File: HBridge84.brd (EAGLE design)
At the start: 53.3 x 40.6 mm, 21 parts, among them J5 ICSP

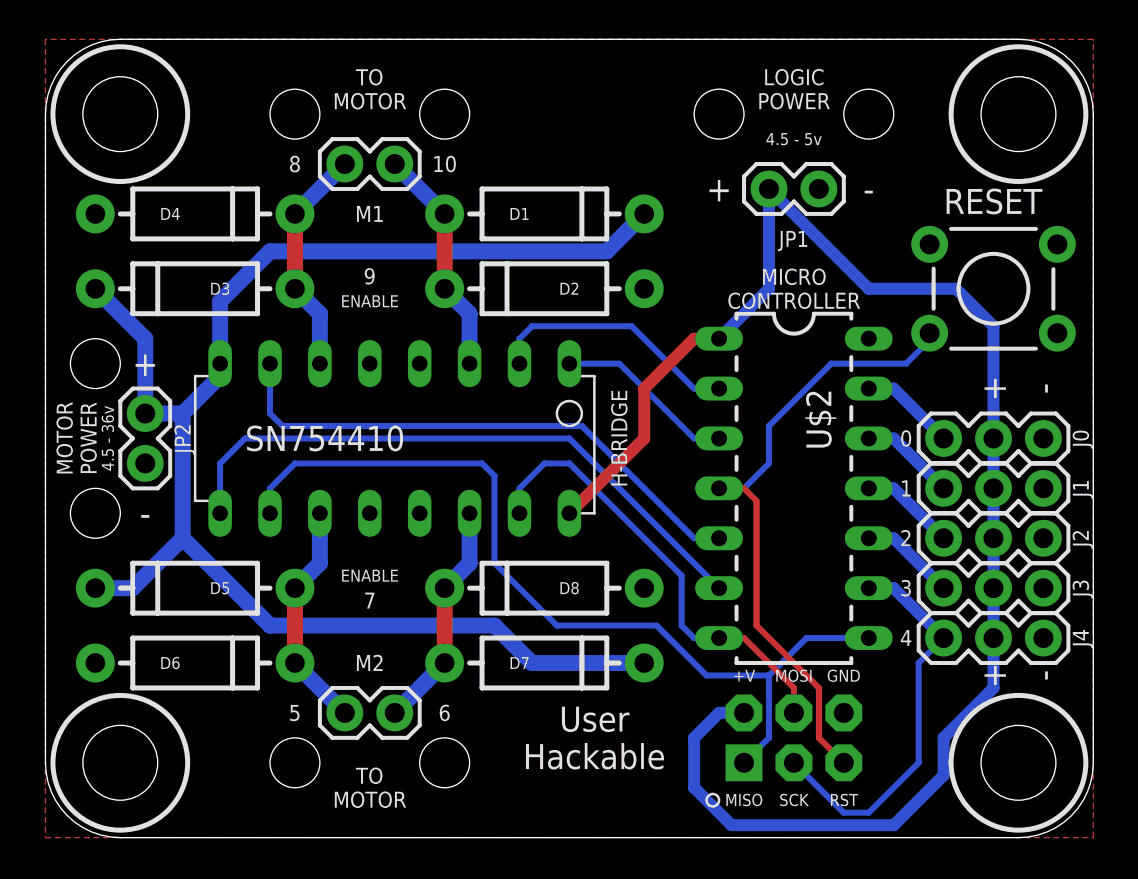
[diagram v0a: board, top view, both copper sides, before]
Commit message: adding eagle files
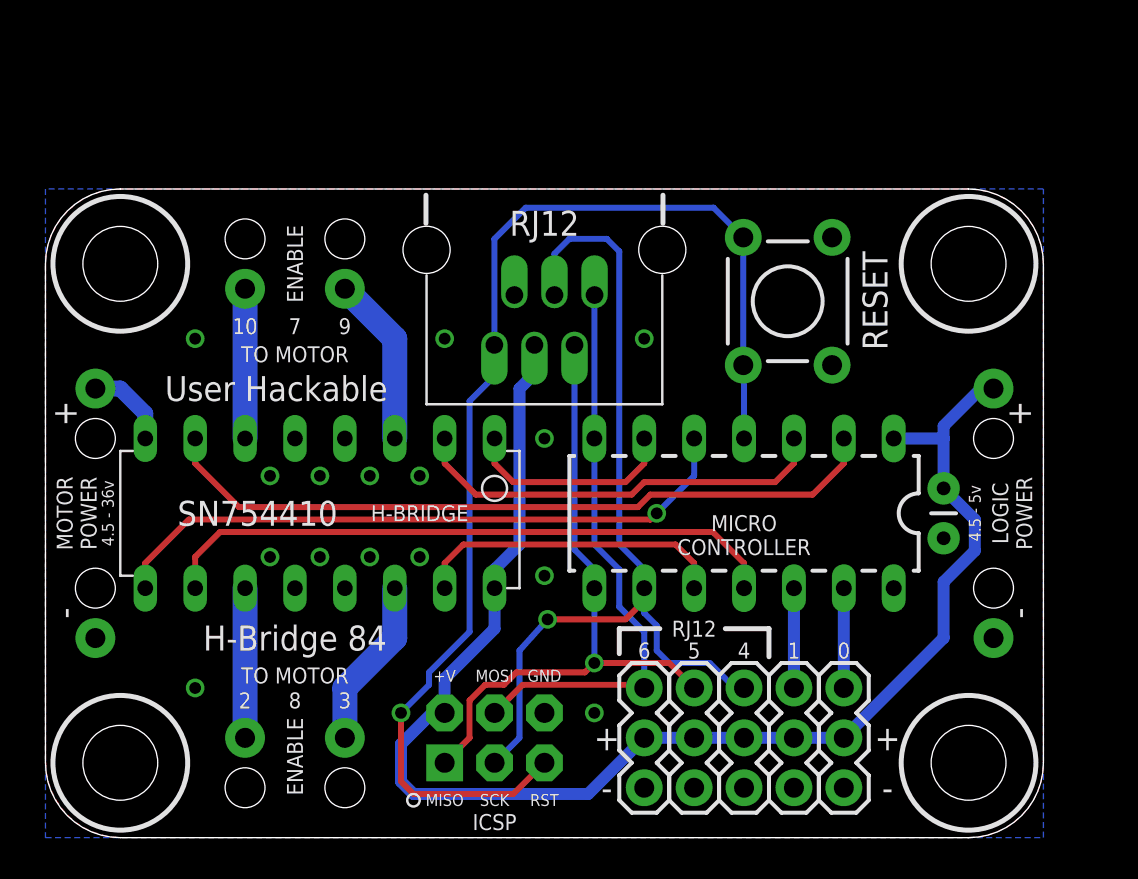
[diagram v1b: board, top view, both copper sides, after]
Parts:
- removed D1, D2, D3, D4, D5, D6, D7, D8: (no value), SparkFun-DiscreteSemi:DIODE-1N4001
- removed JP1, JP2, M1, M2: (no value), SparkFun-Connectors:1X02
- added C2: (no value), barbary_enterprises:CAP-PTH-SMALL
- added U$1, U$10, U$3, U$4, U$5, U$6, U$8, U$9: M1, barbary_enterprises:M1_NO_STRAIN
- added U$7: RJ12, barbary_enterprises:RJ12
- moved J4 21.7 mm to (30.5, 2.54), turned to 90 degrees
- moved J0 20.5 mm to (40.6, 2.54), turned to 90 degrees
- moved J3 20.5 mm to (33.0, 2.54), turned to 90 degrees
- moved J1 19.8 mm to (38.1, 2.54), turned to 90 degrees
- moved J2 19.8 mm to (35.6, 2.54), turned to 90 degrees
- moved J5 15.2 mm to (22.9, 5.08)
- moved RESET 10.5 mm to (37.8, 27.3), turned to 270 degrees
- moved SN754410 5.39 mm to (14.0, 16.5)
- moved U$2 3.81 mm to (34.3, 16.5), turned to 180 degrees
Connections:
- net 10: now also SN754410.7; no longer SN754410.2
- net 2: now also SN754410.10; no longer J2.3
- net 3: now also SN754410.15; no longer J3.3
- net 4: now also J2.3, U$7.4; no longer J4.3
- net 5: now also J3.3, U$7.5; no longer SN754410.10
- net 5V: now also C2.1, U$10.P$1, U$7.3; no longer JP1.2
- net 6: now also J4.3, U$7.6; no longer SN754410.15
- net 7: now also SN754410.1; no longer SN754410.9
- net 8: now also SN754410.9; no longer SN754410.7
- net 9: now also SN754410.2; no longer SN754410.1
- net GND: now also C2.2, RESET.1, U$7.2, U$8.P$1, U$9.P$1; no longer D2.A, D4.A, D6.A, D8.A, JP1.1, JP2.1
- net OUT1: now also U$1.P$1; no longer D1.A, D2.C, M1.2
- net OUT2: now also U$3.P$1; no longer D3.A, D4.C, M1.1
- net OUT3: now also U$4.P$1; no longer D5.A, D6.C, M2.1
- net OUT4: now also U$5.P$1; no longer D7.A, D8.C, M2.2
- net RST: now also RESET.4, U$7.1
- net V_BATT: now also U$6.P$1; no longer D1.C, D3.C, D5.C, D7.C, JP2.2
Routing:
- net V_BATT: track 77.2 -> 4.34 mm
- net RST: track 32.7 -> 62.0 mm, vias 0 -> 1
- net 2: track 4.86 -> 32.0 mm
- net 4: track 20.2 -> 46.6 mm, vias 0 -> 1
- net 10: track 13.0 -> 37.4 mm
- net 7: track 31.6 -> 10.9 mm
- net 9: track 9.20 -> 21.6 mm
- net 5: track 45.1 -> 33.1 mm, vias 0 -> 1
- net 3: track 4.86 -> 16.0 mm
- net 6: track 23.3 -> 29.3 mm
- net 5V: track 79.8 -> 74.6 mm
- net 8: track 28.0 -> 33.0 mm, vias 0 -> 1
- net OUT3: track 11.7 -> 7.62 mm
- net OUT2: track 11.7 -> 7.62 mm
- net OUT4: track 11.7 -> 8.67 mm
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- added copper zone on layer 16, net GND
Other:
- board size 53.3 x 40.6 mm -> 50.8 x 33 mm
- board text added: "H-Bridge 84"
- board text added: "ICSP"
- board text added: "RJ12"
- board text added: "RJ12 and ICSP share pins 4,5,6 and Reset"
